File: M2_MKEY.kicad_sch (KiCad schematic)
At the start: 15 parts, among them J1007 Bus_M.2_Socket_M

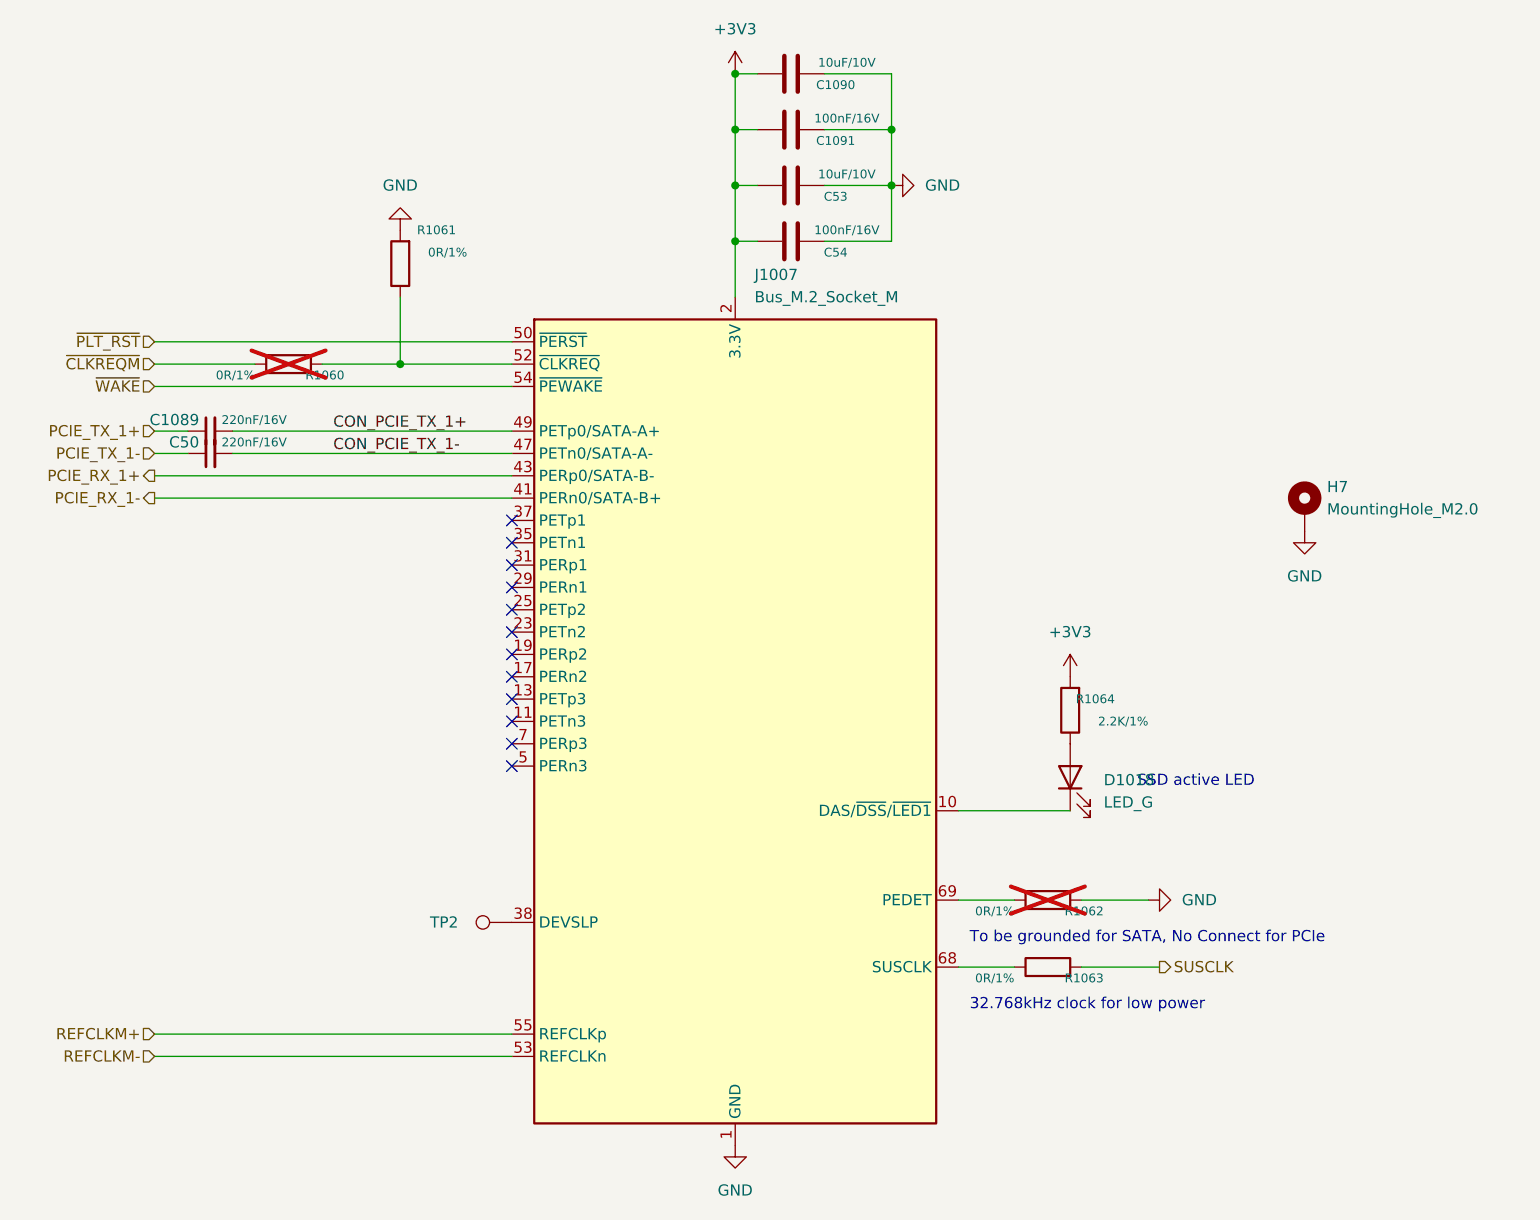
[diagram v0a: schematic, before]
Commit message: commit before removing duplicated glasgow
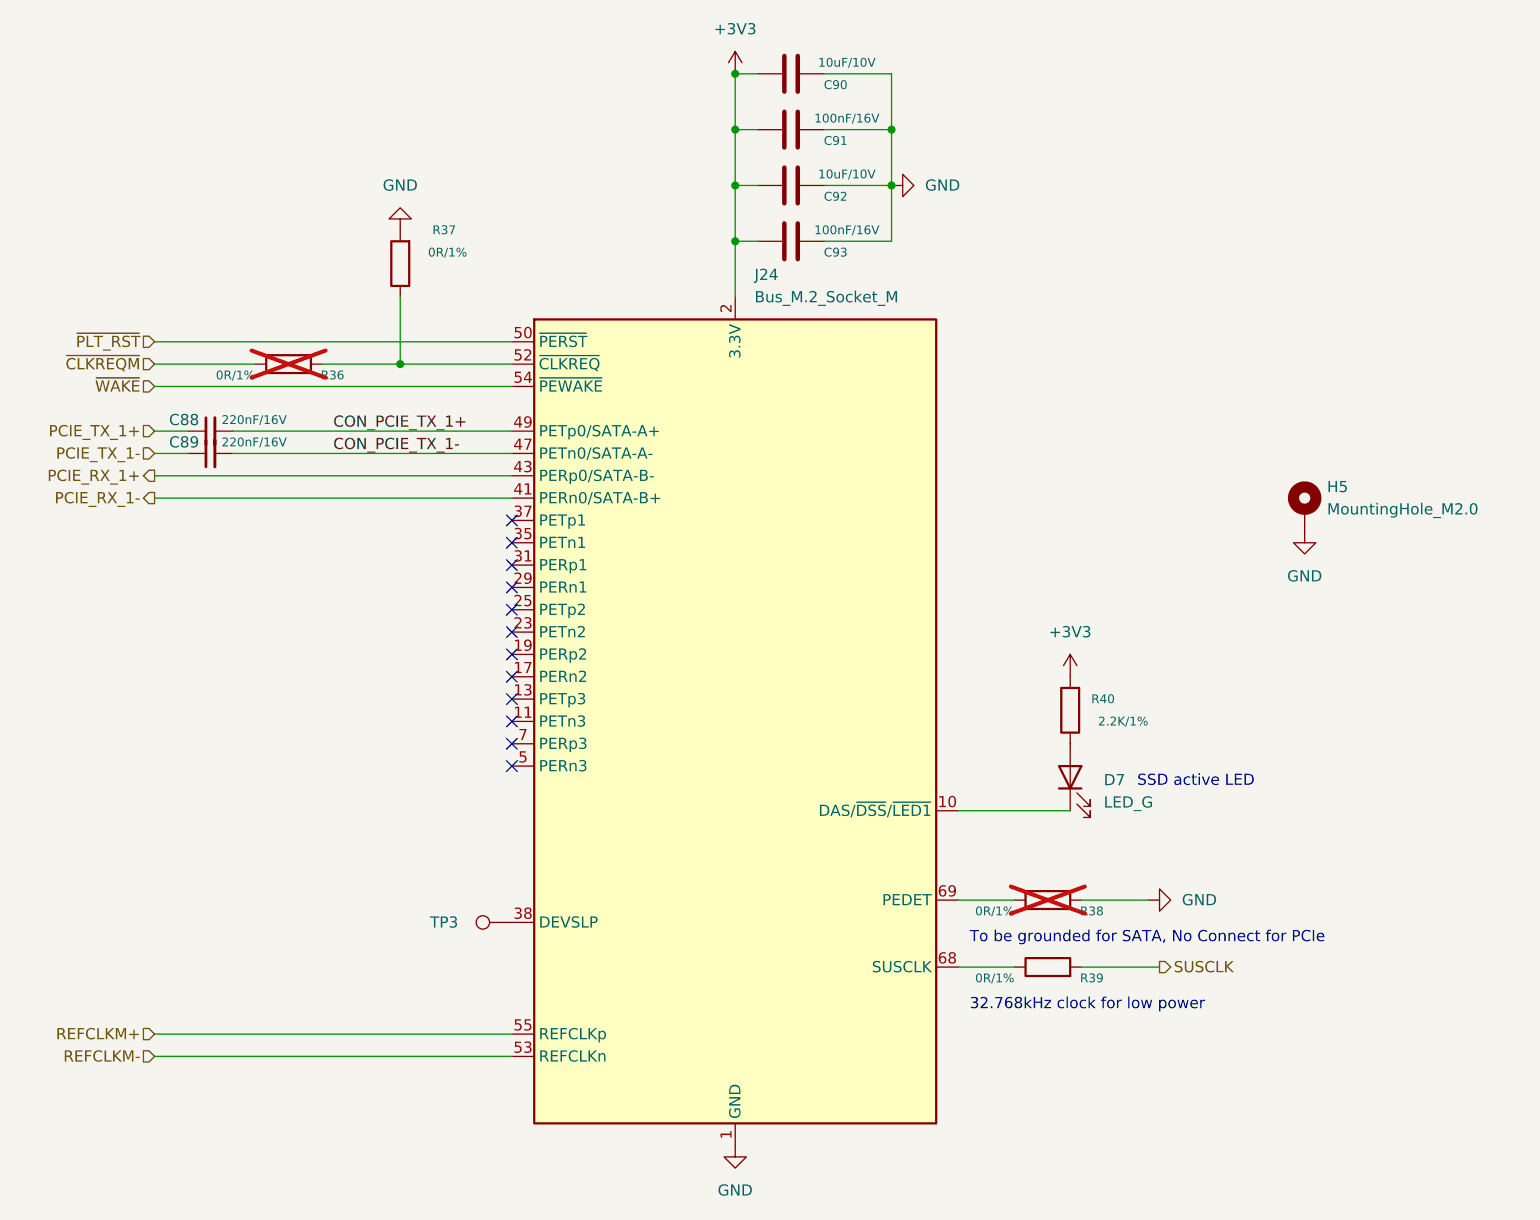
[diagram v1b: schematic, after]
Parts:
- H5: renamed from H7; footprint A_HDJ_Library:MountingHole_2.75mm_M2_4.4mm_Pad_TopOnly -> MountingHole:MountingHole_2.7mm_Pad_TopOnly
- renumbered C1089 to C88, C50 to C89, C1090 to C90, C1091 to C91, C53 to C92, C54 to C93, D1018 to D7, J1007 to J24, R1060 to R36, R1061 to R37, R1062 to R38, R1063 to R39, R1064 to R40, TP2 to TP3
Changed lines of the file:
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@@
 		(on_board yes)
 		(dnp no)
-		(property "Reference" "C1091"
+		(property "Reference" "C91"
 			(at 139.7 34.29 90)
 			(effects
@@
 			(project "microcyber"
 				(path "/7ac319af-771c-4997-a005-b73a4a9b44ab/0f85bef4-33ba-41bd-b468-8a14848b6d64"
-					(reference "C1091")
+					(reference "C91")
 					(unit 1)
 				)
@@
 		(dnp no)
 		(fields_autoplaced yes)
-		(property "Reference" "#PWR01075"
+		(property "Reference" "#PWR096"
 			(at 128.27 30.48 0)
 			(effects
@@
 			(project "microcyber"
 				(path "/7ac319af-771c-4997-a005-b73a4a9b44ab/0f85bef4-33ba-41bd-b468-8a14848b6d64"
-					(reference "#PWR01075")
+					(reference "#PWR096")
 					(unit 1)
 				)
@@
 		(on_board yes)
 		(dnp no)
-		(property "Reference" "R1064"
+		(property "Reference" "R40"
 			(at 171.45 97.79 0)
 			(effects
@@
 			(project "microcyber"
 				(path "/7ac319af-771c-4997-a005-b73a4a9b44ab/0f85bef4-33ba-41bd-b468-8a14848b6d64"
-					(reference "R1064")
+					(reference "R40")
 					(unit 1)
 				)
@@
 		(on_board yes)
 		(dnp no)
-		(property "Reference" "C1089"
+		(property "Reference" "C88"
 			(at 67.31 66.04 90)
 			(effects
@@
 			(project "microcyber"
 				(path "/7ac319af-771c-4997-a005-b73a4a9b44ab/0f85bef4-33ba-41bd-b468-8a14848b6d64"
-					(reference "C1089")
+					(reference "C88")
 					(unit 1)
 				)
@@
 		(dnp no)
 		(fields_autoplaced yes)
-		(property "Reference" "D1018"
+		(property "Reference" "D7"
 			(at 170.18 106.9975 90)
 			(effects
@@
 			(project "microcyber"
 				(path "/7ac319af-771c-4997-a005-b73a4a9b44ab/0f85bef4-33ba-41bd-b468-8a14848b6d64"
-					(reference "D1018")
+					(reference "D7")
 					(unit 1)
 				)
@@
 		(on_board no)
 		(dnp yes)
-		(property "Reference" "R1062"
+		(property "Reference" "R38"
 			(at 170.18 121.92 90)
 			(effects
@@
 			(project "microcyber"
 				(path "/7ac319af-771c-4997-a005-b73a4a9b44ab/0f85bef4-33ba-41bd-b468-8a14848b6d64"
-					(reference "R1062")
+					(reference "R38")
 					(unit 1)
 				)
@@
 		(on_board yes)
 		(dnp no)
-		(property "Reference" "C50"
+		(property "Reference" "C89"
 			(at 67.31 68.58 90)
 			(effects
@@
 			(project "microcyber"
 				(path "/7ac319af-771c-4997-a005-b73a4a9b44ab/0f85bef4-33ba-41bd-b468-8a14848b6d64"
-					(reference "C50")
+					(reference "C89")
 					(unit 1)
 				)
@@
 		(on_board yes)
 		(dnp yes)
-		(property "Reference" "R1060"
+		(property "Reference" "R36"
 			(at 83.82 60.96 90)
 			(effects
@@
 			(project "microcyber"
 				(path "/7ac319af-771c-4997-a005-b73a4a9b44ab/0f85bef4-33ba-41bd-b468-8a14848b6d64"
-					(reference "R1060")
+					(reference "R36")
 					(unit 1)
 				)
@@
 		(on_board yes)
 		(dnp no)
-		(property "Reference" "C53"
+		(property "Reference" "C92"
 			(at 139.7 40.64 90)
 			(effects
@@
 			(project "microcyber"
 				(path "/7ac319af-771c-4997-a005-b73a4a9b44ab/0f85bef4-33ba-41bd-b468-8a14848b6d64"
-					(reference "C53")
+					(reference "C92")
 					(unit 1)
 				)
@@
 		(dnp no)
 		(fields_autoplaced yes)
-		(property "Reference" "#PWR01080"
+		(property "Reference" "#PWR0101"
 			(at 193.04 85.09 0)
 			(effects
@@
 			(project "microcyber"
 				(path "/7ac319af-771c-4997-a005-b73a4a9b44ab/0f85bef4-33ba-41bd-b468-8a14848b6d64"
-					(reference "#PWR01080")
+					(reference "#PWR0101")
 					(unit 1)
 				)
@@
 		(dnp no)
 		(fields_autoplaced yes)
-		(property "Reference" "J1007"
+		(property "Reference" "J24"
 			(at 130.4641 49.53 0)
 			(effects
@@
 			(project "microcyber"
 				(path "/7ac319af-771c-4997-a005-b73a4a9b44ab/0f85bef4-33ba-41bd-b468-8a14848b6d64"
-					(reference "J1007")
+					(reference "J24")
 					(unit 1)
 				)
@@
 		(dnp no)
 		(fields_autoplaced yes)
-		(property "Reference" "#PWR01078"
+		(property "Reference" "#PWR099"
 			(at 166.37 99.06 0)
 			(effects
@@
 			(project "microcyber"
 				(path "/7ac319af-771c-4997-a005-b73a4a9b44ab/0f85bef4-33ba-41bd-b468-8a14848b6d64"
-					(reference "#PWR01078")
+					(reference "#PWR099")
 					(unit 1)
 				)
@@
 		(dnp no)
 		(fields_autoplaced yes)
-		(property "Reference" "#PWR01077"
+		(property "Reference" "#PWR098"
 			(at 152.4 39.37 0)
 			(effects
@@
 			(project "microcyber"
 				(path "/7ac319af-771c-4997-a005-b73a4a9b44ab/0f85bef4-33ba-41bd-b468-8a14848b6d64"
-					(reference "#PWR01077")
+					(reference "#PWR098")
 					(unit 1)
 				)
@@
 		(dnp no)
 		(fields_autoplaced yes)
-		(property "Reference" "#PWR01079"
+		(property "Reference" "#PWR0100"
 			(at 181.61 120.65 0)
 			(effects
@@
 			(project "microcyber"
 				(path "/7ac319af-771c-4997-a005-b73a4a9b44ab/0f85bef4-33ba-41bd-b468-8a14848b6d64"
-					(reference "#PWR01079")
+					(reference "#PWR0100")
 					(unit 1)
 				)
@@
 		(on_board yes)
 		(dnp no)
-		(property "Reference" "TP2"
+		(property "Reference" "TP3"
 			(at 96.774 123.19 90)
 			(effects
@@
 			(project "microcyber"
 				(path "/7ac319af-771c-4997-a005-b73a4a9b44ab/0f85bef4-33ba-41bd-b468-8a14848b6d64"
-					(reference "TP2")
+					(reference "TP3")
 					(unit 1)
 				)
@@
 		(dnp no)
 		(fields_autoplaced yes)
-		(property "Reference" "#PWR01076"
+		(property "Reference" "#PWR097"
 			(at 128.27 154.94 0)
 			(effects
@@
 			(project "microcyber"
 				(path "/7ac319af-771c-4997-a005-b73a4a9b44ab/0f85bef4-33ba-41bd-b468-8a14848b6d64"
-					(reference "#PWR01076")
+					(reference "#PWR097")
 					(unit 1)
 				)
@@
 		(dnp no)
 		(fields_autoplaced yes)
-		(property "Reference" "H7"
+		(property "Reference" "H5"
 			(at 195.58 73.66 0)
 			(effects
@@
 			)
 		)
-		(property "Footprint" "A_HDJ_Library:MountingHole_2.75mm_M2_4.4mm_Pad_TopOnly"
+		(property "Footprint" "MountingHole:MountingHole_2.7mm_Pad_TopOnly"
 			(at 193.04 76.2 0)
 			(effects
@@
 			(project "microcyber"
 				(path "/7ac319af-771c-4997-a005-b73a4a9b44ab/0f85bef4-33ba-41bd-b468-8a14848b6d64"
-					(reference "H7")
+					(reference "H5")
 					(unit 1)
 				)
@@
 		(dnp no)
 		(fields_autoplaced yes)
-		(property "Reference" "#PWR01074"
+		(property "Reference" "#PWR095"
 			(at 90.17 38.1 0)
 			(effects
@@
 			(project "microcyber"
 				(path "/7ac319af-771c-4997-a005-b73a4a9b44ab/0f85bef4-33ba-41bd-b468-8a14848b6d64"
-					(reference "#PWR01074")
+					(reference "#PWR095")
 					(unit 1)
 				)
@@
 		(on_board yes)
 		(dnp no)
-		(property "Reference" "C54"
+		(property "Reference" "C93"
 			(at 139.7 46.99 90)
 			(effects
@@
 			(project "microcyber"
 				(path "/7ac319af-771c-4997-a005-b73a4a9b44ab/0f85bef4-33ba-41bd-b468-8a14848b6d64"
-					(reference "C54")
+					(reference "C93")
 					(unit 1)
 				)
@@
 		(on_board yes)
 		(dnp no)
-		(property "Reference" "C1090"
+		(property "Reference" "C90"
 			(at 139.7 27.94 90)
 			(effects
@@
 			(project "microcyber"
 				(path "/7ac319af-771c-4997-a005-b73a4a9b44ab/0f85bef4-33ba-41bd-b468-8a14848b6d64"
-					(reference "C1090")
+					(reference "C90")
 					(unit 1)
 				)
@@
 		(on_board yes)
 		(dnp no)
-		(property "Reference" "R1061"
+		(property "Reference" "R37"
 			(at 96.52 44.45 0)
 			(effects
@@
 			(project "microcyber"
 				(path "/7ac319af-771c-4997-a005-b73a4a9b44ab/0f85bef4-33ba-41bd-b468-8a14848b6d64"
-					(reference "R1061")
+					(reference "R37")
 					(unit 1)
 				)
@@
 		(on_board yes)
 		(dnp no)
-		(property "Reference" "R1063"
+		(property "Reference" "R39"
 			(at 170.18 129.54 90)
 			(effects
@@
 			(project "microcyber"
 				(path "/7ac319af-771c-4997-a005-b73a4a9b44ab/0f85bef4-33ba-41bd-b468-8a14848b6d64"
-					(reference "R1063")
-					(unit 1)
-				)
+					(reference "R39")
+					(unit 1)
+				)
